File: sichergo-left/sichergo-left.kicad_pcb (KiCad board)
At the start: 2 copper layers, 111.8 x 103.2 mm, 117 parts, among them J1 Conn_01x04_Pin, Q1 2N7002, SW1 SW_Push, SW10 SW_Push, SW11 SW_Push, SW12 SW_Push, SW13 SW_Push, SW14 SW_Push, SW15 SW_Push, SW16 SW_Push, SW17 SW_Push, SW18 SW_Push, SW19 MS-22C01-G010, SW2 SW_Push, SW3 SW_Push, SW4 SW_Push, SW5 SW_Push, SW6 SW_Push, SW7 SW_Push, SW8 SW_Push, SW9 SW_Push, U1 AZ1117-3.3, U2 TPD4E05U06DQA, U3 YTS1C0033BBG01, U4 STM32F103C8Tx, U5 SN74LVC1G125DBV, U6 SN74LVC1G125DBV, Y1 Crystal_GND24

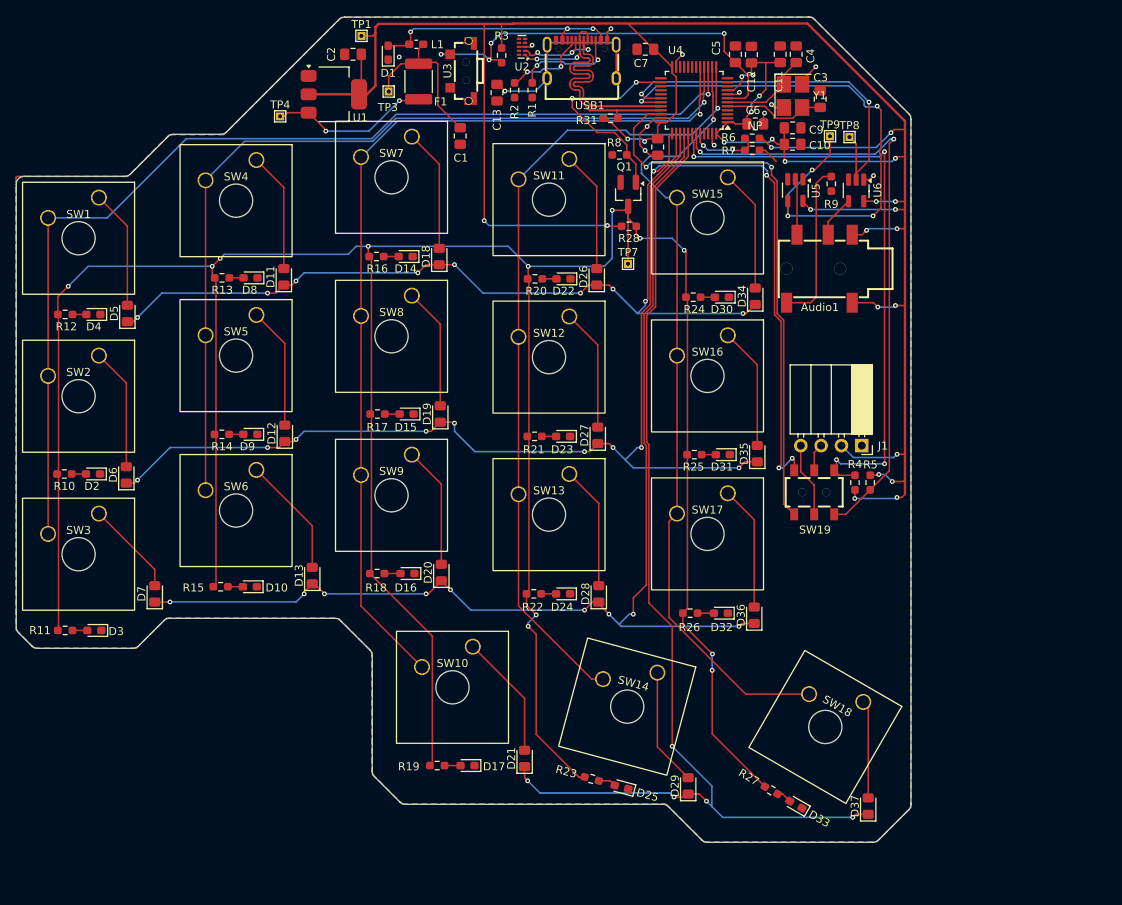
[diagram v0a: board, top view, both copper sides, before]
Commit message: Remake entire shape
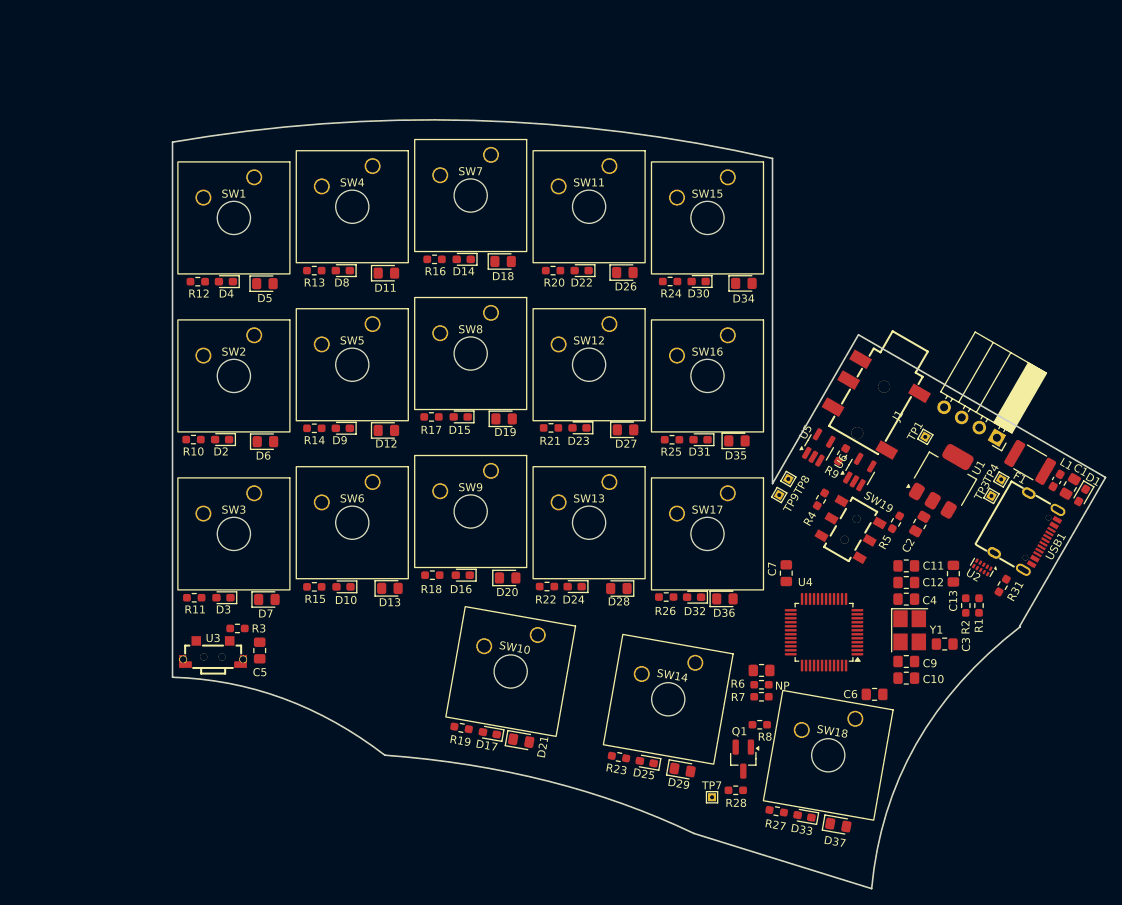
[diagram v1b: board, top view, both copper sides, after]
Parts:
- moved D1 102.9 mm to (223.7, 111.1), turned to -120 degrees
- moved TP4 100.9 mm to (213.6, 109.1), turned to 60 degrees
- moved L1 96.9 mm to (220.6, 109.3), turned to 60 degrees
- moved C5 95.3 mm to (120.9, 130.5), turned to -90 degrees
- moved C2 92.0 mm to (203.4, 114.7), turned to -120 degrees
- moved TP3 90.7 mm to (212.4, 111.2), turned to 60 degrees
- moved U1 90.3 mm to (206.6, 109.1), turned to 60 degrees
- moved F1 90.1 mm to (217.2, 107.0), turned to 150 degrees
- moved C1 87.9 mm to (222.2, 110.0), turned to -120 degrees
- moved U2 86.9 mm to (211.3, 120.1), turned to -120 degrees
- moved TP1 86.5 mm to (204.1, 103.8), turned to 60 degrees
- moved R2 85.6 mm to (209.2, 124.9)
- moved R1 85.3 mm to (210.8, 124.9)
- moved C13 82.9 mm to (207.7, 120.9)
- moved USB1 81.3 mm to (217.0, 115.8), turned to -120 degrees
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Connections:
- R28 pad 1: /MatrixL/LED_DRIVE -> +3V3
- R28 pad 2: +3V3 -> /MatrixL/LED_DRIVE
- U4 pad 18: unconnected-(U4-PB0-Pad18) -> /KB_ROW_1
- U4 pad 19: unconnected-(U4-PB1-Pad19) -> /KB_ROW_2
- U4 pad 20: unconnected-(U4-PB2-Pad20) -> /KB_ROW_3
- U4 pad 21: unconnected-(U4-PB10-Pad21) -> /KB_ROW_0
- U4 pad 38: /KB_ROW_0 -> unconnected-(U4-PA15-Pad38)
- U4 pad 39: /KB_ROW_1 -> unconnected-(U4-PB3-Pad39)
- U4 pad 40: /KB_ROW_2 -> unconnected-(U4-PB4-Pad40)
- U4 pad 41: /KB_ROW_3 -> unconnected-(U4-PB5-Pad41)
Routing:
- net /MatrixL/LED_DRIVE: track 385.0 -> 0.00 mm, vias 12 -> 0
- net +3V3: track 336.5 -> 0.00 mm, vias 27 -> 0
- net /KB_ROW_2: track 145.4 -> 0.00 mm, vias 9 -> 0
- net /KB_ROW_3: track 136.0 -> 0.00 mm, vias 5 -> 0
- net /KB_COL_0: track 131.8 -> 0.00 mm, vias 1 -> 0
- net /KB_ROW_1: track 130.0 -> 0.00 mm, vias 9 -> 0
- net /KB_COL_2: track 117.4 -> 0.00 mm, vias 1 -> 0
- net /KB_ROW_0: track 109.8 -> 0.00 mm, vias 9 -> 0
- net /KB_COL_1: track 109.6 -> 0.00 mm, vias 1 -> 0
- net /KB_COL_3: track 102.0 -> 0.00 mm, vias 1 -> 0
- net /KB_COL_4: track 99.3 -> 0.00 mm, vias 1 -> 0
- net /OLED_SDA: track 78.4 -> 0.00 mm, vias 2 -> 0
- net /OLED_SCL: track 76.2 -> 0.00 mm, vias 4 -> 0
- net /UART_RX: track 73.5 -> 0.00 mm, vias 5 -> 0
- net /SWDIO: track 70.3 -> 0.00 mm, vias 2 -> 0
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- removed copper zone on B.Cu, net GND
- removed copper zone on F.Cu, net GND
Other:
- board size 111.8 x 103.2 mm -> 116.6 x 96.1 mm
- board text added: "Daniel (steewBSD)"
